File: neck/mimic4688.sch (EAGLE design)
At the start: 56 parts, among them J1 JST-VH-3, P1 44PINEDGE, Q1 2N3906, Q10 2N3906, Q2 2N3906, Q3 2N3906, Q4 2N3904, Q5 2N3904, Q6 2N3904, Q7 2N3904, Q8 2N3906, Q9 2N3906

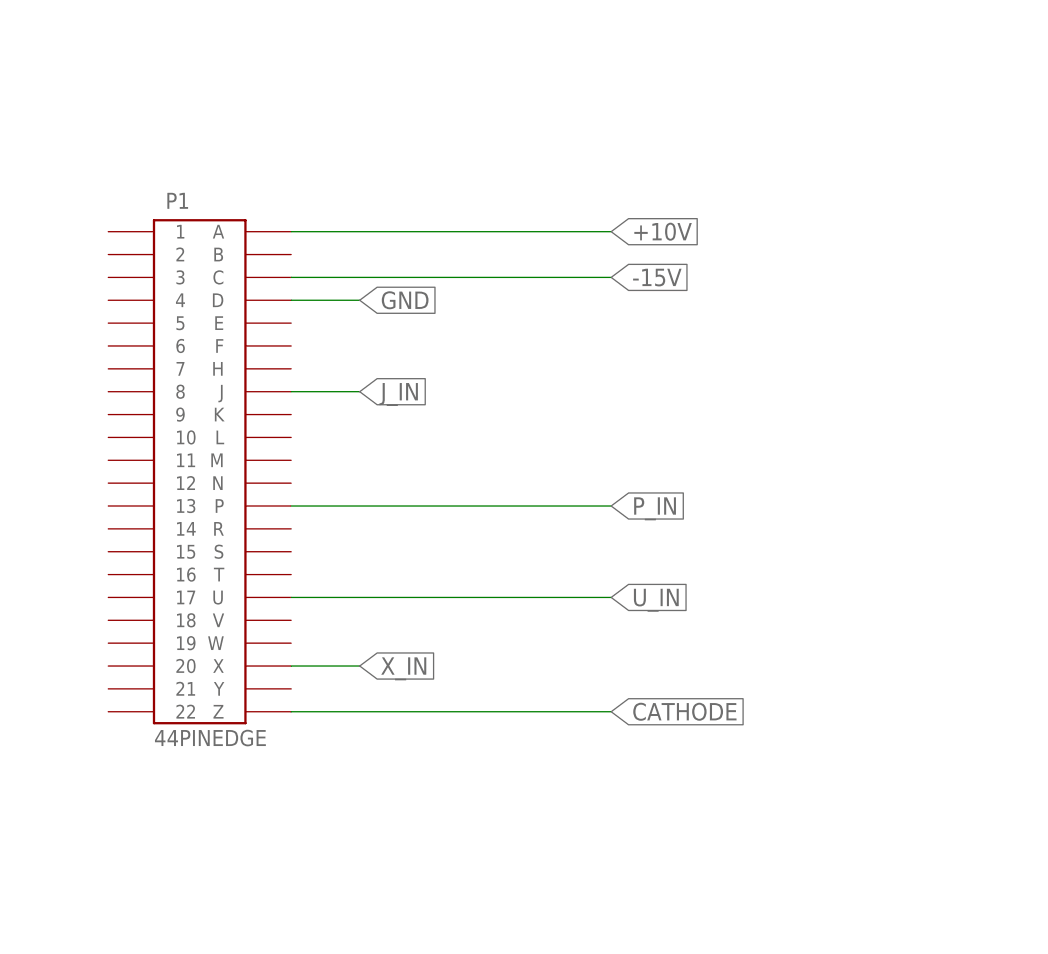
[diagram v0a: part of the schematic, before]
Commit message: revised artwork
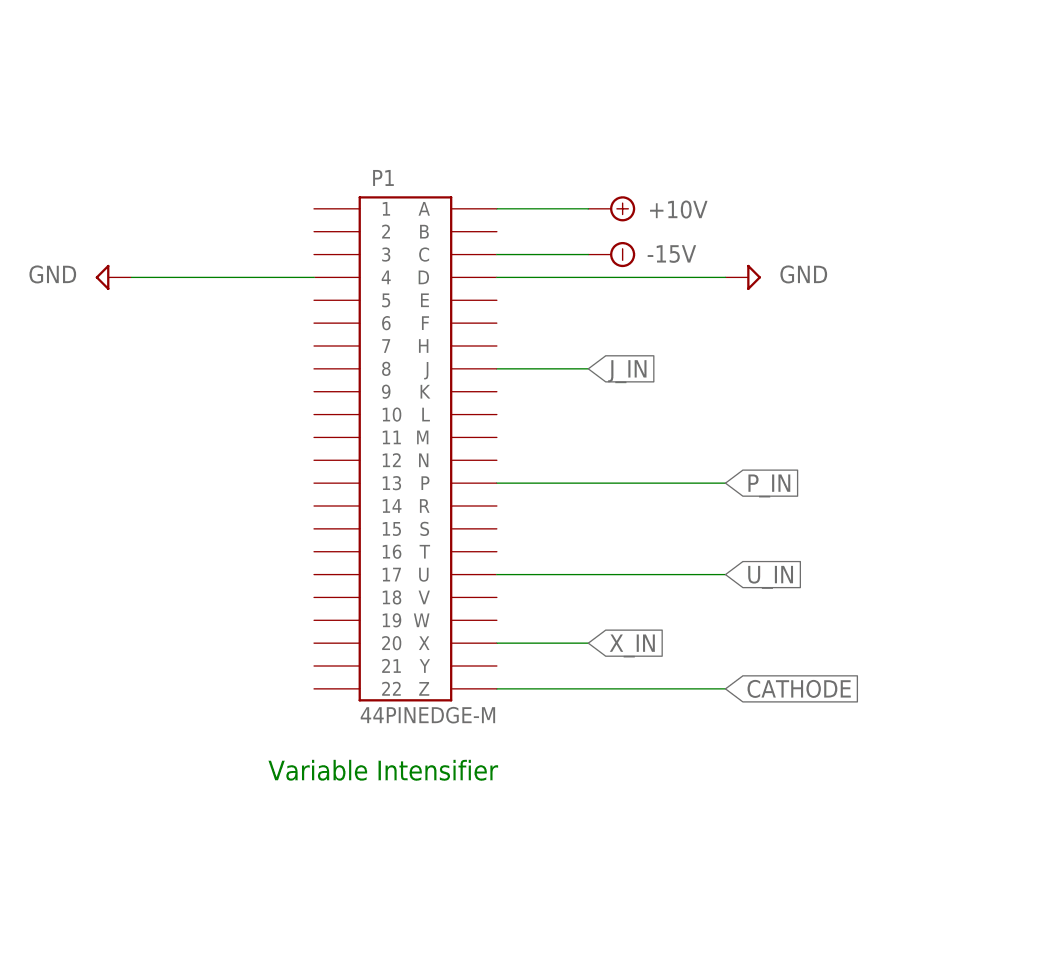
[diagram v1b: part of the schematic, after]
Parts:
- P1: value 44PINEDGE -> 44PINEDGE-M; device keiths:44PINEDGE -> keiths:44PINEDGE-M
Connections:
- net GND: now also P1.4
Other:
- note added: "Variable Intensifier"
- moved on the sheet: P1
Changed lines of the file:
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@@
 <part name="FRAME1" library="frames" deviceset="FRAME_C_L" device=""/>
 <part name="FRAME2" library="frames" deviceset="FRAME_C_L" device=""/>
-<part name="P1" library="keiths" deviceset="44PINEDGE" device=""/>
 <part name="SUPPLY1" library="keiths" deviceset="GND" device=""/>
 <part name="R28" library="keiths" deviceset="R-1/4WATT" device="" value="11.3K"/>
@@
 <part name="R16" library="keiths" deviceset="R-1/4WATT" device="" value="23.7K"/>
 <part name="D5" library="keiths" deviceset="1N4148" device="" value="1N4148"/>
+<part name="U$2" library="adafruit" deviceset="FIDUCIAL" device=""/>
 <part name="U$1" library="adafruit" deviceset="FIDUCIAL" device=""/>
-<part name="U$2" library="adafruit" deviceset="FIDUCIAL" device=""/>
+<part name="P1" library="keiths" deviceset="44PINEDGE-M" device=""/>
+<part name="SUPPLY40" library="keiths" deviceset="GND" device=""/>
+<part name="SUPPLY45" library="keiths" deviceset="GND" device=""/>
+<part name="SUPPLY46" library="keiths" deviceset="-15V" device=""/>
+<part name="SUPPLY47" library="supply2" deviceset="+10V" device=""/>
 </parts>
 <sheets>
@@
 <text x="459.74" y="195.58" size="3.81" layer="91" font="vector" ratio="10">Connector to
 mimic1705 bias.</text>
+<text x="73.66" y="180.34" size="2.1844" layer="91" font="vector" ratio="10">Variable Intensifier</text>
 </plain>
 <instances>
 <instance part="FRAME1" gate="G$1" x="0" y="0"/>
 <instance part="FRAME2" gate="G$2" x="452.12" y="0"/>
-<instance part="P1" gate="G$1" x="66.04" y="215.9"/>
 <instance part="SUPPLY1" gate="GND" x="368.3" y="358.14" rot="MR180"/>
 <instance part="R28" gate="&gt;NAME" x="226.06" y="96.52" smashed="yes" rot="MR90">
@@
 <attribute name="VALUE" x="320.04" y="226.06" size="1.9304" layer="96" font="vector" ratio="10"/>
 </instance>
-<instance part="U$1" gate="G$1" x="485.14" y="398.78"/>
-<instance part="U$2" gate="G$1" x="500.38" y="398.78"/>
+<instance part="U$2" gate="G$1" x="485.14" y="398.78"/>
+<instance part="U$1" gate="G$1" x="500.38" y="398.78"/>
+<instance part="P1" gate="G$1" x="88.9" y="218.44"/>
+<instance part="SUPPLY40" gate="GND" x="55.88" y="236.22" smashed="yes" rot="MR90">
+<attribute name="VALUE" x="52.451" y="235.585" size="1.9304" layer="96" font="vector" ratio="10" rot="MR0"/>
+</instance>
+<instance part="SUPPLY45" gate="GND" x="127" y="236.22" smashed="yes" rot="R90">
+<attribute name="VALUE" x="130.429" y="235.585" size="1.9304" layer="96" font="vector" ratio="10"/>
+</instance>
+<instance part="SUPPLY46" gate="G$1" x="111.76" y="238.76" smashed="yes" rot="R90">
+<attribute name="VALUE" x="115.697" y="237.871" size="1.9304" layer="96" font="vector" ratio="10"/>
+</instance>
+<instance part="SUPPLY47" gate="G$1" x="111.76" y="243.84" smashed="yes" rot="MR90">
+<attribute name="VALUE" x="115.824" y="244.729" size="1.9304" layer="96" font="vector" ratio="10" rot="MR180"/>
+</instance>
 </instances>
 <busses>
@@
 </segment>
 <segment>
-<pinref part="P1" gate="G$1" pin="D"/>
-<wire x1="76.2" y1="233.68" x2="83.82" y2="233.68" width="0.1524" layer="91"/>
-<label x="83.82" y="233.68" size="1.9304" layer="95" font="vector" ratio="10" xref="yes"/>
-</segment>
-<segment>
 <wire x1="436.88" y1="200.66" x2="429.26" y2="200.66" width="0.1524" layer="91"/>
 <wire x1="429.26" y1="200.66" x2="429.26" y2="190.5" width="0.1524" layer="91"/>
@@
 <wire x1="210.82" y1="274.32" x2="210.82" y2="281.94" width="0.1524" layer="91"/>
 </segment>
+<segment>
+<wire x1="99.06" y1="236.22" x2="124.46" y2="236.22" width="0.1524" layer="91"/>
+<pinref part="SUPPLY45" gate="GND" pin="GND"/>
+<pinref part="P1" gate="G$1" pin="D"/>
+</segment>
+<segment>
+<pinref part="SUPPLY40" gate="GND" pin="GND"/>
+<wire x1="58.42" y1="236.22" x2="78.74" y2="236.22" width="0.1524" layer="91"/>
+<pinref part="P1" gate="G$1" pin="4"/>
+</segment>
 </net>
 <net name="J_IN" class="0">
@@
 </segment>
 <segment>
+<label x="109.22" y="226.06" size="1.9304" layer="95" font="vector" ratio="10" xref="yes"/>
 <pinref part="P1" gate="G$1" pin="J"/>
-<wire x1="76.2" y1="223.52" x2="83.82" y2="223.52" width="0.1524" layer="91"/>
-<label x="83.82" y="223.52" size="1.9304" layer="95" font="vector" ratio="10" xref="yes"/>
+<wire x1="99.06" y1="226.06" x2="109.22" y2="226.06" width="0.1524" layer="91"/>
 </segment>
 </net>
@@
 </segment>
 <segment>
-<pinref part="P1" gate="G$1" pin="C"/>
-<wire x1="76.2" y1="236.22" x2="111.76" y2="236.22" width="0.1524" layer="91"/>
-<label x="111.76" y="236.22" size="1.9304" layer="95" font="vector" ratio="10" xref="yes"/>
-</segment>
-<segment>
 <label x="185.42" y="114.3" size="1.9304" layer="95" font="vector" ratio="10" rot="MR0" xref="yes"/>
 <pinref part="Q9" gate="G$1" pin="C"/>
@@
 <wire x1="226.06" y1="162.56" x2="226.06" y2="160.02" width="0.1524" layer="91"/>
 <junction x="226.06" y="160.02"/>
+</segment>
+<segment>
+<pinref part="SUPPLY46" gate="G$1" pin="-15V"/>
+<pinref part="P1" gate="G$1" pin="C"/>
+<wire x1="99.06" y1="238.76" x2="109.22" y2="238.76" width="0.1524" layer="91"/>
 </segment>
 </net>
@@
 </segment>
 <segment>
+<label x="124.46" y="203.2" size="1.9304" layer="95" font="vector" ratio="10" xref="yes"/>
 <pinref part="P1" gate="G$1" pin="U"/>
-<wire x1="76.2" y1="200.66" x2="111.76" y2="200.66" width="0.1524" layer="91"/>
-<label x="111.76" y="200.66" size="1.9304" layer="95" font="vector" ratio="10" xref="yes"/>
+<wire x1="99.06" y1="203.2" x2="124.46" y2="203.2" width="0.1524" layer="91"/>
 </segment>
 </net>
@@
 </segment>
 <segment>
+<label x="109.22" y="195.58" size="1.9304" layer="95" font="vector" ratio="10" xref="yes"/>
 <pinref part="P1" gate="G$1" pin="X"/>
-<wire x1="76.2" y1="193.04" x2="83.82" y2="193.04" width="0.1524" layer="91"/>
-<label x="83.82" y="193.04" size="1.9304" layer="95" font="vector" ratio="10" xref="yes"/>
+<wire x1="99.06" y1="195.58" x2="109.22" y2="195.58" width="0.1524" layer="91"/>
 </segment>
 </net>
@@
 </segment>
 <segment>
+<label x="124.46" y="213.36" size="1.9304" layer="95" font="vector" ratio="10" xref="yes"/>
 <pinref part="P1" gate="G$1" pin="P"/>
-<wire x1="76.2" y1="210.82" x2="111.76" y2="210.82" width="0.1524" layer="91"/>
-<label x="111.76" y="210.82" size="1.9304" layer="95" font="vector" ratio="10" xref="yes"/>
+<wire x1="99.06" y1="213.36" x2="124.46" y2="213.36" width="0.1524" layer="91"/>
 </segment>
 </net>
@@
 <net name="+10V" class="0">
 <segment>
-<pinref part="P1" gate="G$1" pin="A"/>
-<wire x1="76.2" y1="241.3" x2="111.76" y2="241.3" width="0.1524" layer="91"/>
-<label x="111.76" y="241.3" size="1.9304" layer="95" font="vector" ratio="10" xref="yes"/>
-</segment>
-<segment>
 <pinref part="R28" gate="&gt;NAME" pin="P$1"/>
 <wire x1="226.06" y1="106.68" x2="226.06" y2="101.6" width="0.1524" layer="91"/>
@@
 <pinref part="R16" gate="&gt;NAME" pin="P$1"/>
 <wire x1="264.16" y1="205.74" x2="241.3" y2="205.74" width="0.1524" layer="91"/>
+</segment>
+<segment>
+<pinref part="SUPPLY47" gate="G$1" pin="+10V"/>
+<pinref part="P1" gate="G$1" pin="A"/>
+<wire x1="99.06" y1="243.84" x2="109.22" y2="243.84" width="0.1524" layer="91"/>
 </segment>
 </net>
@@
 </segment>
 <segment>
-<wire x1="76.2" y1="187.96" x2="111.76" y2="187.96" width="0.1524" layer="91"/>
-<label x="111.76" y="187.96" size="1.9304" layer="95" font="vector" ratio="10" xref="yes"/>
+<wire x1="99.06" y1="190.5" x2="124.46" y2="190.5" width="0.1524" layer="91"/>
+<label x="124.46" y="190.5" size="1.9304" layer="95" font="vector" ratio="10" xref="yes"/>
 <pinref part="P1" gate="G$1" pin="Z"/>
 </segment>
